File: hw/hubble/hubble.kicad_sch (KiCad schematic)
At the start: 39 parts

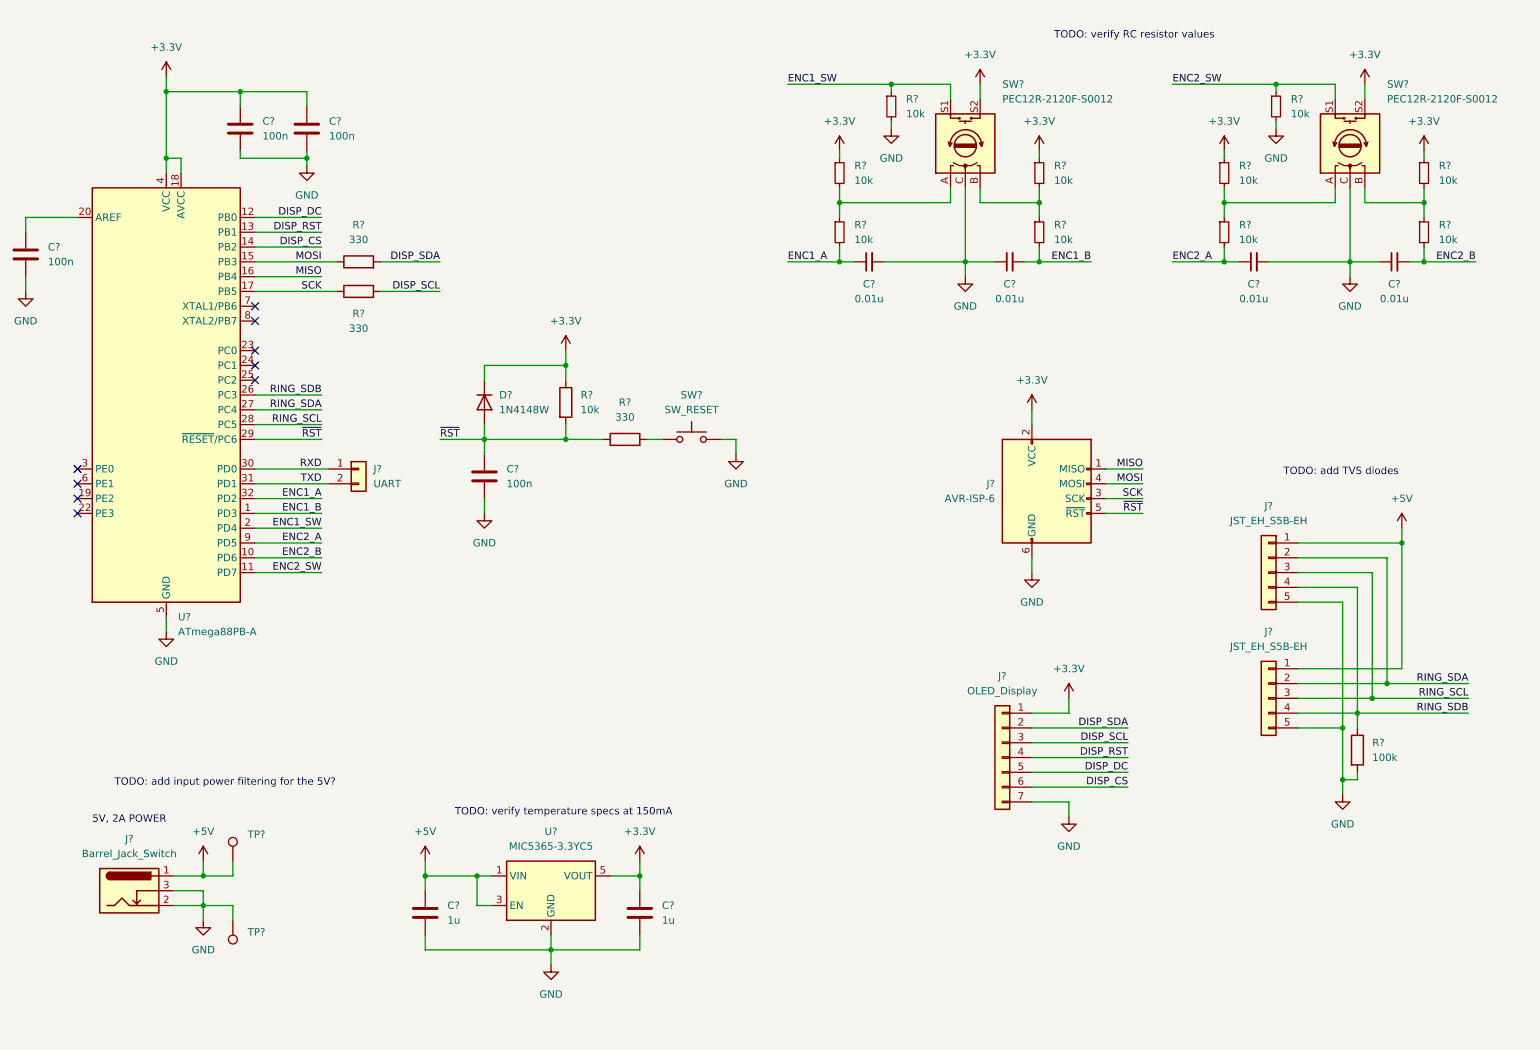
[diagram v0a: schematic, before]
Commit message: Start initial hubble layout
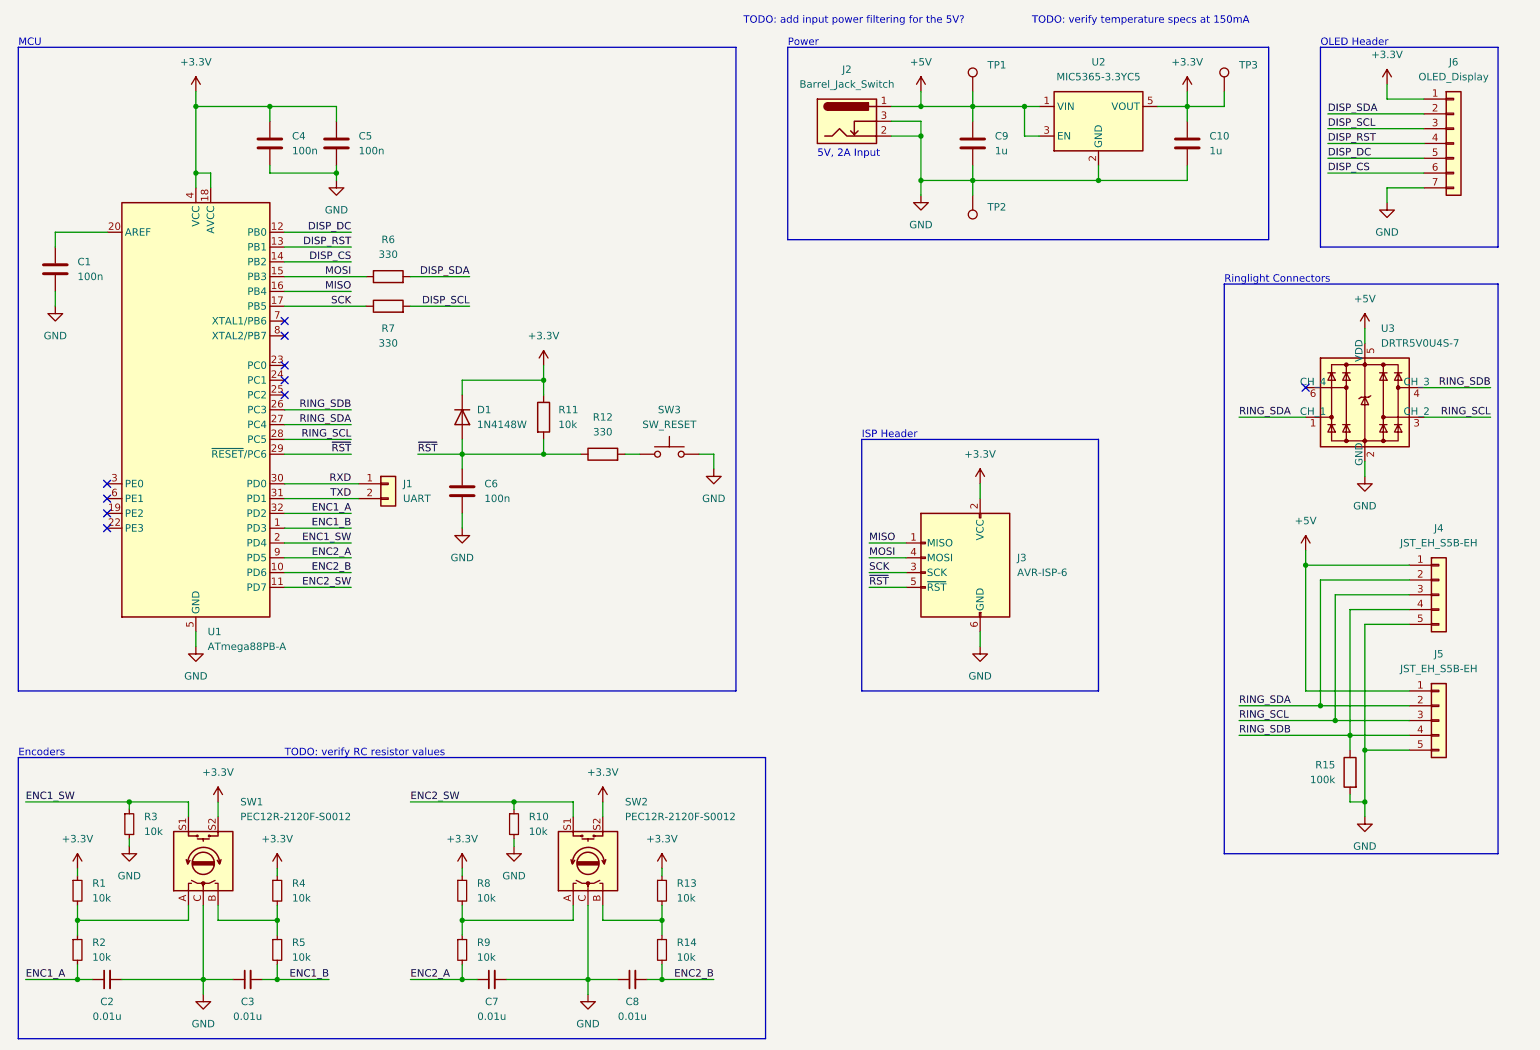
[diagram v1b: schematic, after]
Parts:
- added TP3: TestPoint, TestPoint:TestPoint_THTPad_D2.0mm_Drill1.0mm, symbol Connector:TestPoint
- added U3: DRTR5V0U4S-7, Package_TO_SOT_SMD:SOT-363_SC-70-6, symbol earendel:DRTR5V0U4S-7
- C10, C9: renamed from C?; footprint (none) -> Capacitor_SMD:C_0805_2012Metric
- R10, R3: renamed from R?; footprint (none) -> Resistor_SMD:R_0805_2012Metric
- SW1, SW2: renamed from SW?; footprint (none) -> earendel:PEC12R-2120F-S0012
- TP1, TP2: renamed from TP?; footprint (none) -> TestPoint:TestPoint_THTPad_D2.0mm_Drill1.0mm
- gave numbers to parts that had none: 31
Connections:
- net +3.3V: now also TP3.1
- net +5V: now also U3.5 (VDD)
- net GND: now also U3.2 (GND)
- net RING_SCL: now also U3.3 (CH_2)
- net RING_SDA: now also U3.1 (CH_1)
- net RING_SDB: now also U3.4 (CH_3)
- no-connect marks 9 -> 10
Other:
- note added: "5V, 2A Input"
- note added: "Encoders"
- note added: "ISP Header"
- note added: "MCU"
- note added: "OLED Header"
- note added: "Power"
- note added: "Ringlight Connectors"
- note removed: "5V, 2A POWER"
- note removed: "TODO: add TVS diodes"
- moved on the sheet: C1, C10, C2, C3, C4, C5, C6, C7, C8, C9, D1, J1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
